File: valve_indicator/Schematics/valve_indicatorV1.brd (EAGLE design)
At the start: 93.3 x 95.1 mm, 130 parts, among them Q1 PMV45EN2R, Q2 PMV45EN2R, Q3 PMV45EN2R, Q4 PMV45EN2R, Q5 IRF9530, Q6 PMV45EN2R, U1 MC33063ADR, U2 MC33063ADR, U3 STM32F103RET6, X1 ECS-160-10-36Q-ES-TR_16MHZ

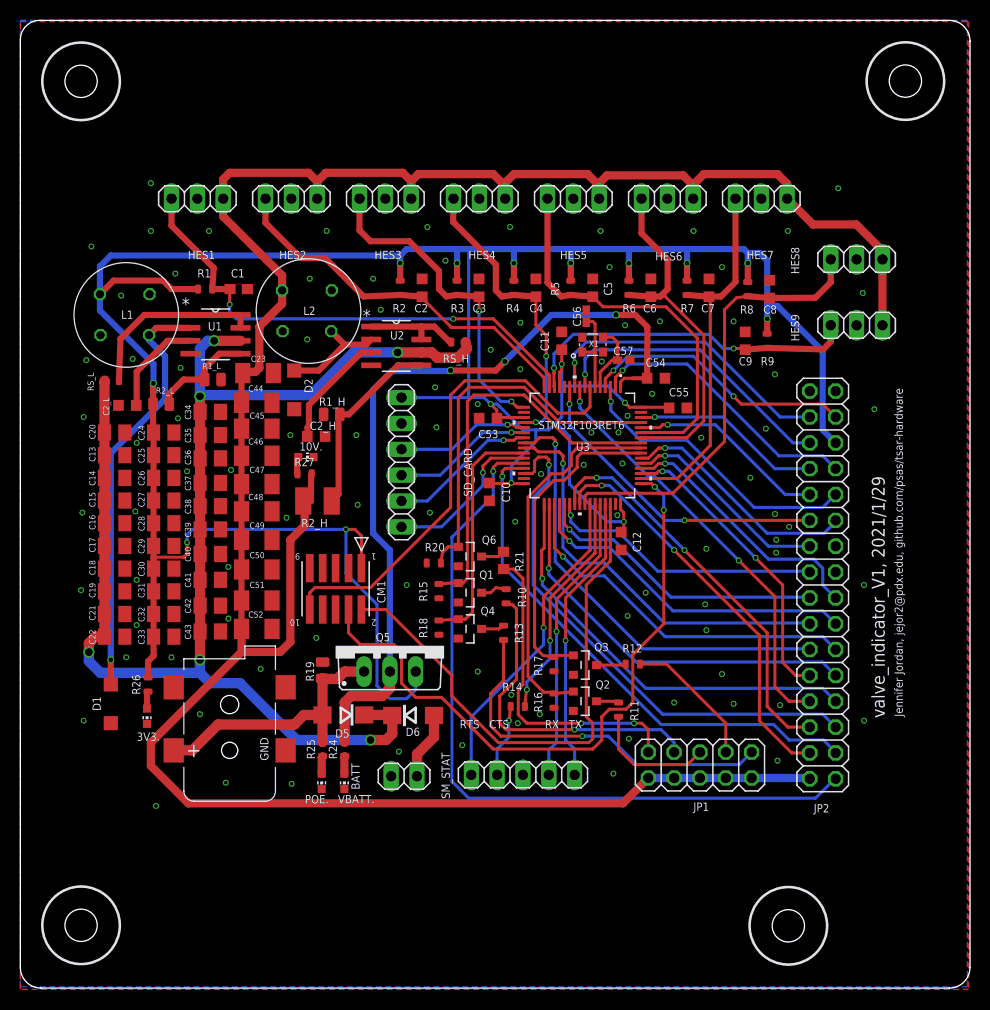
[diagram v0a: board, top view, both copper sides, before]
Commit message: Vi changes
Added SD card circuit. Added 9POS for sending position sensor data to the SFE board. Updated attributes.
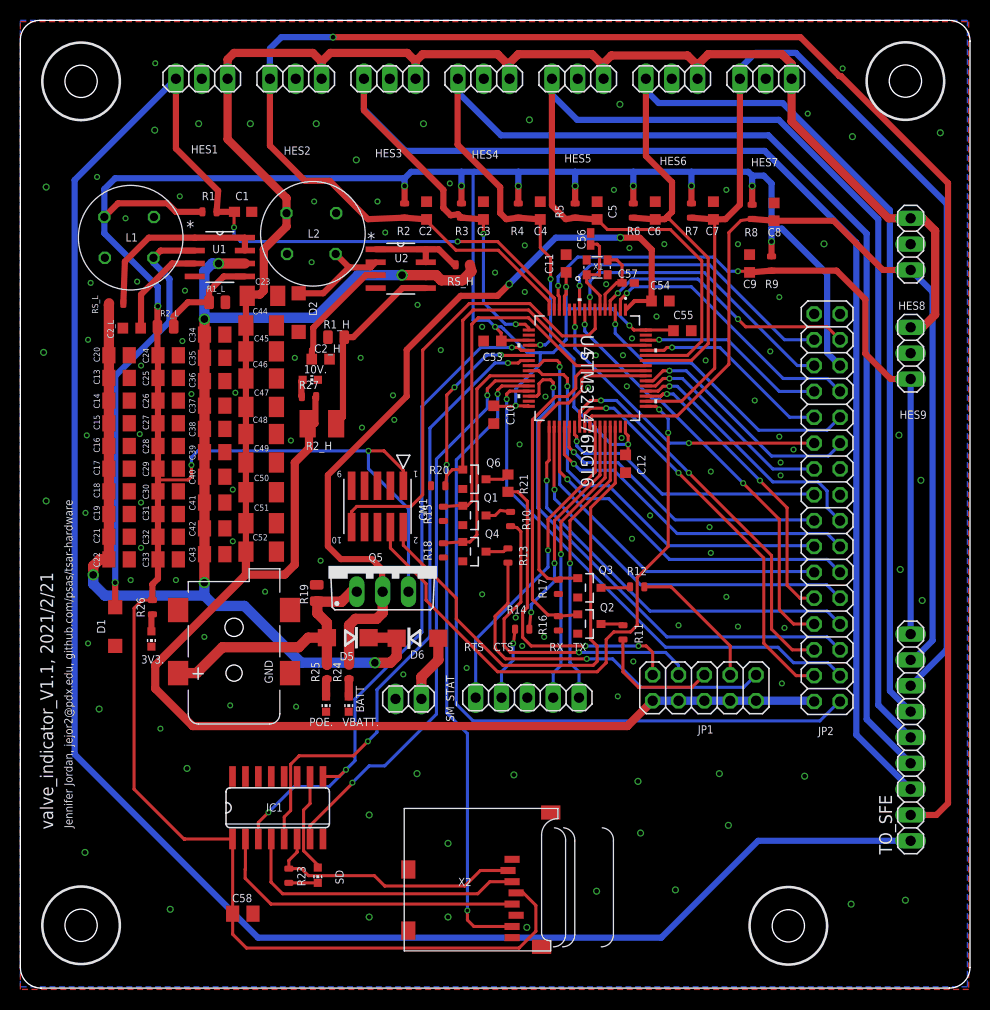
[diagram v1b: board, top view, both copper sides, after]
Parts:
- removed SD_CARD: SD, pinhead:1X06
- removed U3: STM32F103RET6, STM32F103RET6:LQFP64-10X10MM
- added C58: 10uF, oresat-rcl:C0805K
- added IC1: (no value), 40xx:SO16
- added R23: 1k, oresat-rcl:.0603-C-NOSILK
- added SD: (no value), led:CHIP-LED0603
- added TO_SFE: (no value), pinhead:1X09
- added U4: STM32L476RGT6, STM32L476RGT6:LQFP64-10X10MM_STM
- added X2: (no value), adafruit:MICROSD
- moved HES1 11.8 mm to (17.8, 89.3)
- moved HES2 11.8 mm to (27.1, 89.3)
- moved HES3 11.8 mm to (36.3, 89.3)
- moved HES4 11.8 mm to (45.5, 89.3)
- moved HES5 11.8 mm to (54.8, 89.3)
- moved HES6 11.8 mm to (64.0, 89.3)
- moved HES7 11.8 mm to (73.3, 89.3)
- moved CM1 9.09 mm to (35.1, 47.2)
- moved Q5 7.88 mm to (35.6, 41.4)
- moved R19 7.62 mm to (29.1, 38.7)
- moved C54 7.61 mm to (62.9, 67.4)
- moved D2 7.61 mm to (27.4, 66.3)
- moved R21 7.61 mm to (47.9, 49.5)
- moved RS_H 7.61 mm to (43.5, 71.0)
- moved U2 7.61 mm to (37.4, 70.6)
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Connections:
- new net N$20: IC1.6, R23.1, X2.2
- new net N$22: R23.2, SD.C
- new net N$23: IC1.4, X2.3
- new net N$6: IC1.10, SD.A
- new net N$8: IC1.2, X2.5
- net +3V3: now also C58.1, IC1.1, U4.13, U4.19, U4.32, U4.48, U4.64, X2.4; no longer SD_CARD.6, U3.13, U3.19, U3.32, U3.48, U3.64
- net BOOT0: now also U4.60; no longer U3.60
- net GND: now also C58.2, IC1.11, IC1.14, IC1.8, U4.12, U4.18, U4.31, U4.47, U4.63, X2.6, X2.MT1, X2.MT2; no longer SD_CARD.5, U3.12, U3.18, U3.31, U3.47, U3.63
- net IN_CTS: now also U4.44; no longer U3.44
- net IN_H1: now also TO_SFE.1, U4.15; no longer U3.15
- net IN_H2: now also TO_SFE.2, U4.16; no longer U3.16
- net IN_H3: now also TO_SFE.3, U4.17; no longer U3.17
- net IN_H4: now also TO_SFE.4, U4.20; no longer U3.20
- net IN_H5: now also TO_SFE.5, U4.59; no longer U3.59
- net IN_H6: now also TO_SFE.6, U4.58; no longer U3.58
- net IN_H7: now also TO_SFE.7, U4.50; no longer U3.50
- net IN_H8: now also TO_SFE.8, U4.41; no longer U3.41
- net IN_H9: now also TO_SFE.9, U4.14; no longer U3.14
- net IN_RTS: now also U4.45; no longer U3.45
- net IN_UART-RX: now also U4.43; no longer U3.43
- net IN_UART-TX: now also U4.42; no longer U3.42
- net N$30: now also U4.46; no longer U3.46
- net N$32: now also U4.7; no longer U3.7
- net N$9: now also U4.49; no longer U3.49
- net OSC_IN: now also U4.5; no longer U3.5
- net OSC_OUT: now also U4.6; no longer U3.6
- net OUT_BUZZ: now also U4.26; no longer U3.26
- net OUT_CLK: now also IC1.3, IC1.9, U4.21; no longer SD_CARD.4, U3.21
- net OUT_CS: now also IC1.7, U4.27; no longer SD_CARD.1, U3.27
- net OUT_DI: now also IC1.5, U4.23; no longer SD_CARD.2, U3.23
- net OUT_DO: now also U4.22, X2.7; no longer SD_CARD.3, U3.22
- net OUT_LED0: now also U4.61; no longer U3.61
- net OUT_LED1: now also U4.57; no longer U3.57
- net OUT_LED2: now also U4.56; no longer U3.56
- net OUT_LED3: now also U4.55; no longer U3.55
- net PB10: now also U4.29; no longer U3.29
- net PB11: now also U4.30; no longer U3.30
- net PB12: now also U4.33; no longer U3.33
- net PB13: now also U4.34; no longer U3.34
- net PB14: now also U4.35; no longer U3.35
- net PB15: now also U4.36; no longer U3.36
- net PB2: now also U4.28; no longer U3.28
- net PB9: now also U4.62; no longer U3.62
- net PC0: now also U4.8; no longer U3.8
- net PC1: now also U4.9; no longer U3.9
- net PC10: now also U4.51; no longer U3.51
- net PC11: now also U4.52; no longer U3.52
- net PC12: now also U4.53; no longer U3.53
- net PC13: now also U4.2; no longer U3.2
- net PC14-OSC32_IN: now also U4.3; no longer U3.3
- net PC15-OSC32_OUT: now also U4.4; no longer U3.4
- net PC2: now also U4.10; no longer U3.10
- net PC3: now also U4.11; no longer U3.11
- net PC4: now also U4.24; no longer U3.24
- net PC5: now also U4.25; no longer U3.25
- net PC6: now also U4.37; no longer U3.37
- net PC7: now also U4.38; no longer U3.38
- net PC8: now also U4.39; no longer U3.39
- net PC9: now also U4.40; no longer U3.40
- net PD2: now also U4.54; no longer U3.54
- net VBATT: now also U4.1; no longer U3.1
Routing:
- net IN_H1: track 49.8 -> 218.1 mm
- net IN_H2: track 37.1 -> 182.4 mm, vias 0 -> 1
- net IN_H3: track 32.3 -> 146.9 mm
- net IN_H4: track 29.6 -> 134.9 mm
- net IN_H5: track 39.3 -> 134.4 mm
- net IN_H6: track 36.5 -> 120.8 mm
- net IN_H7: track 36.4 -> 117.5 mm
- net +3V3: track 297.4 -> 363.2 mm
- net OUT_CLK: track 13.1 -> 66.7 mm, vias 1 -> 3
- net OUT_DO: track 13.8 -> 66.8 mm, vias 1 -> 4
- net OUT_DI: track 14.6 -> 61.9 mm, vias 1 -> 2
- net IN_H8: track 43.5 -> 90.3 mm
- net OUT_CS: track 15.9 -> 56.8 mm, vias 1 -> 2
- net IN_H9: track 33.9 -> 72.0 mm
- net N$8: track 0.00 -> 31.2 mm
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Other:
- board text added: "valve_indicator_V1.1, 2021/2/21"
- board text removed: "valve_indicator_V1, 2021/1/29"
